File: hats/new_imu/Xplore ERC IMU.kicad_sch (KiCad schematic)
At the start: 42 parts, among them J1 5025850670, J2 5025850570, SW1 CAS-220TA, U1 LIS3MDL, U2 BMI088, U3 LT3960JMSE-PBF, U4 AMS1117-3.3, U5 D5V0H1B2LP-7B

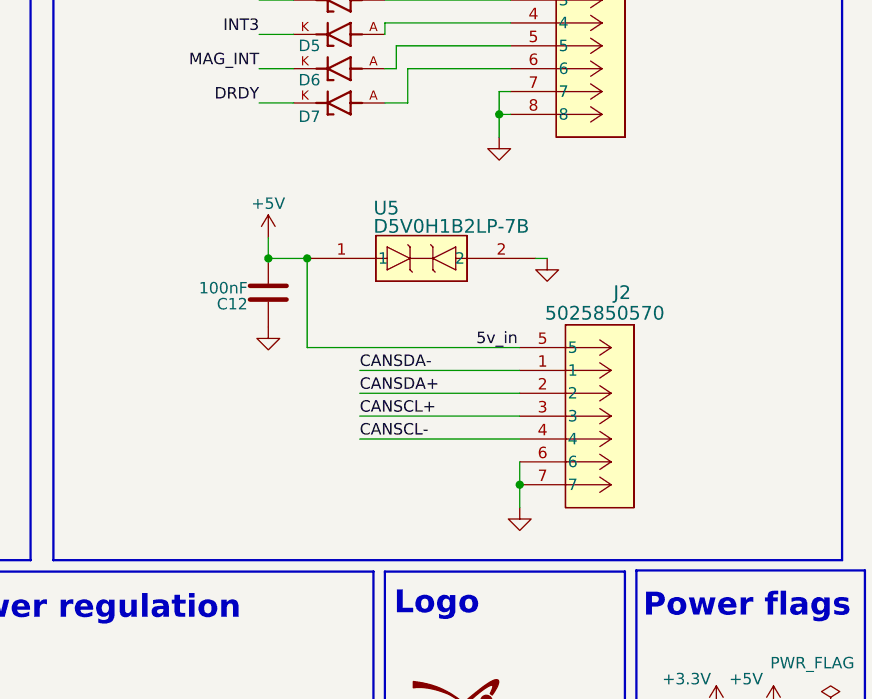
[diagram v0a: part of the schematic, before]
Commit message: IMU Layout and routing fixes
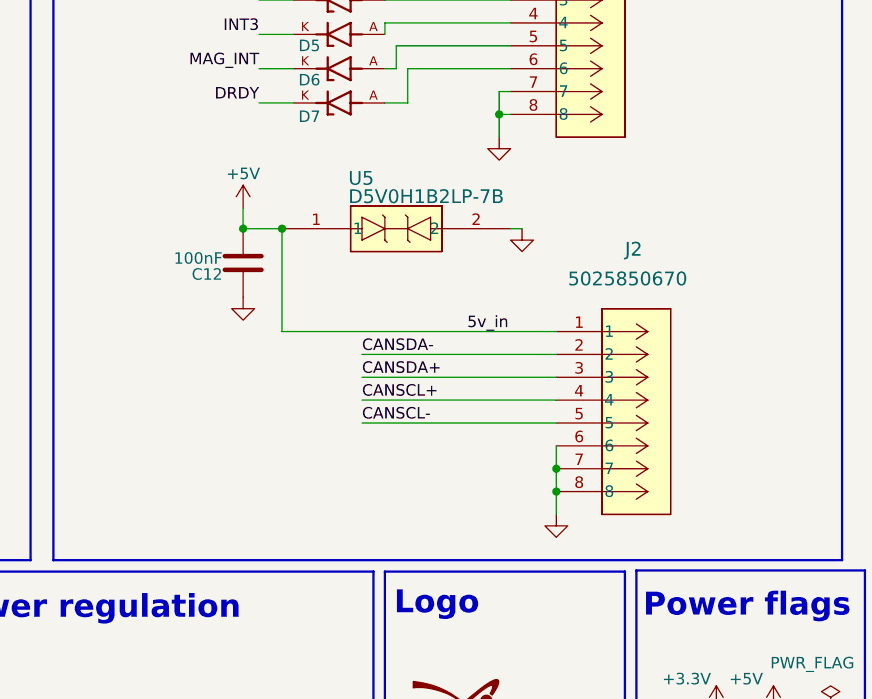
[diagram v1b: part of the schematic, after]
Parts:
- removed J2: 5025850570, footprints:CON_5025850570, symbol 5025850570:5025850570
- added J2: 5025850670, footprints:CON_5025850670, symbol 502585670:5025850670
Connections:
- net +5V: now also J2.1
- net CANSCL+: now also J2.4
- net CANSCL-: now also J2.5
- net CANSDA+: now also J2.3
- net CANSDA-: now also J2.2
- net GND: now also J2.6, J2.7, J2.8
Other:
- moved on the sheet: C12, U5

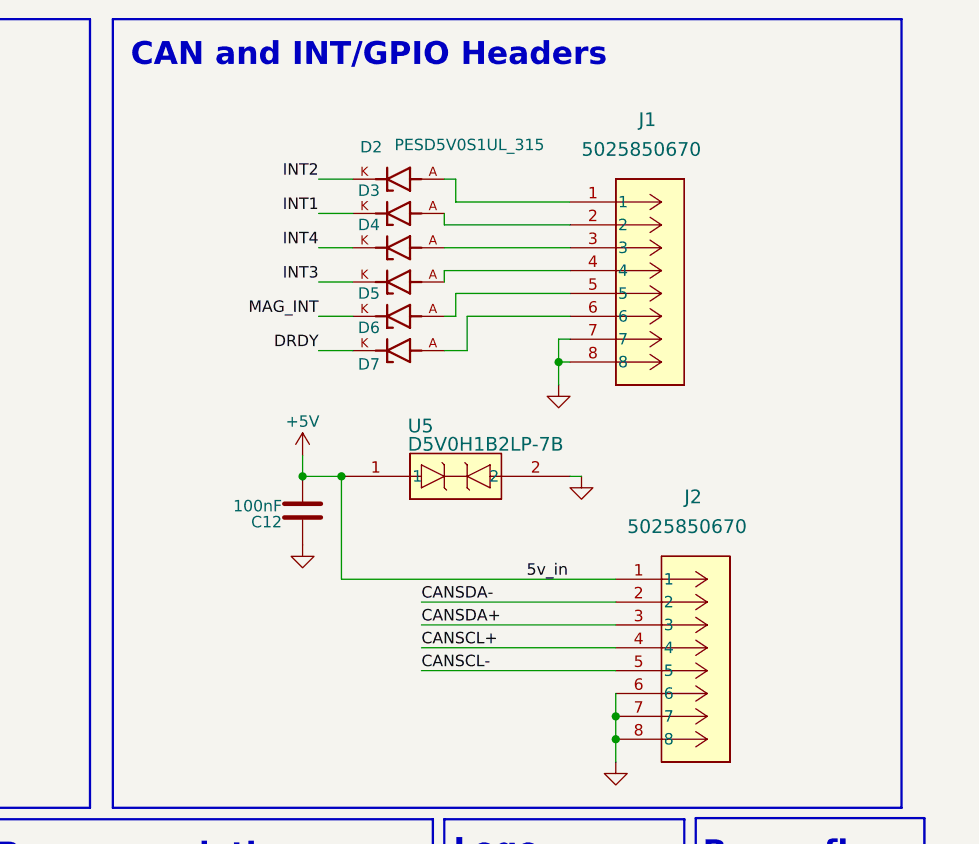
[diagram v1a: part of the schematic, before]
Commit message: IMU tweaks
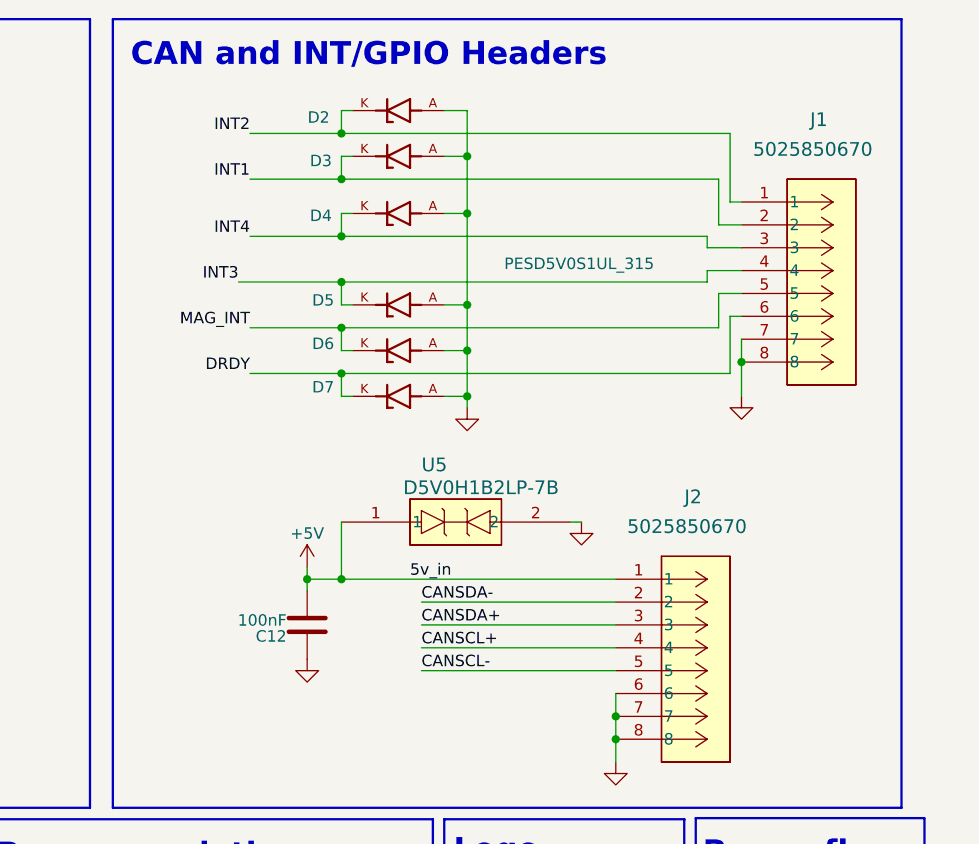
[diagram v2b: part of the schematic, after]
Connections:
- net DRDY: now also J1.6
- net GND: now also D2.A, D3.A, D4.A, D5.A, D6.A, D7.A
- net INT1: now also J1.2
- net INT2: now also J1.1
- net INT3: now also J1.4
- net INT4: now also J1.3
- net MAG_INT: now also J1.5
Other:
- moved on the sheet: C12, D3, D4, D5, D6, D7, J1, U5

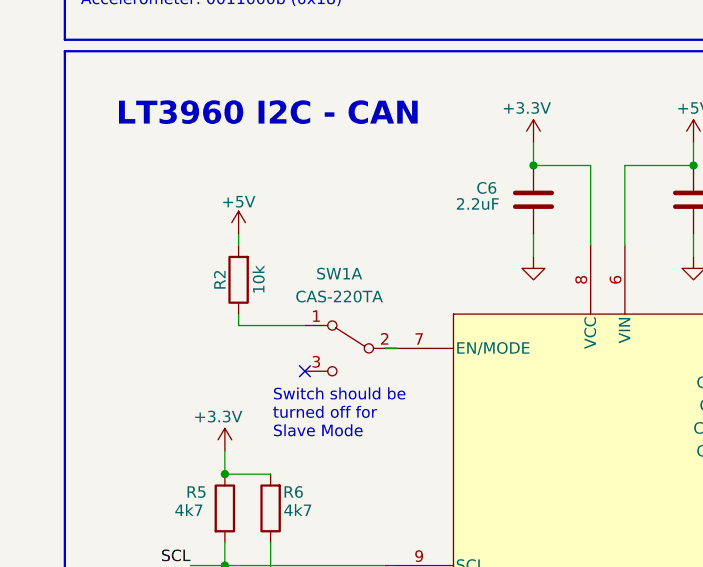
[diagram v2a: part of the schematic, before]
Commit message: IMU final touches
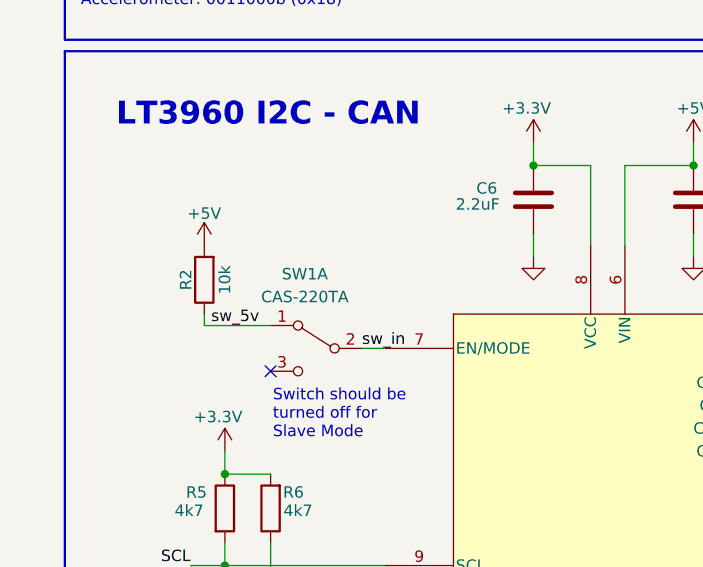
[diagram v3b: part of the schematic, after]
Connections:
- net sw_5v: now reaches R2.1, SW1.1 (A)
- net sw_in: now reaches SW1.2 (B), U3.7 (EN/MODE)
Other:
- moved on the sheet: R2, SW1A
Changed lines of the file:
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@@
 	)
 	(no_connect
-		(at 40.64 144.78)
+		(at 36.83 144.78)
 	)
 	(wire
@@
 	(wire
 		(pts
-			(xy 40.64 139.7) (xy 33.274 139.7)
+			(xy 36.83 139.7) (xy 29.464 139.7)
 		)
 		(stroke
@@
 	(wire
 		(pts
-			(xy 50.8 142.24) (xy 49.53 142.24)
-		)
-		(stroke
-			(width 0)
-			(type default)
-		)
-	)
-	(wire
-		(pts
 			(xy 100.33 148.59) (xy 104.14 148.59)
 		)
@@
 	(wire
 		(pts
-			(xy 33.274 139.7) (xy 33.274 138.43)
+			(xy 29.464 139.7) (xy 29.464 138.43)
 		)
 		(stroke
@@
 	(wire
 		(pts
+			(xy 46.99 142.24) (xy 49.53 142.24)
+		)
+		(stroke
+			(width 0)
+			(type default)
+		)
+	)
+	(wire
+		(pts
 			(xy 220.98 137.16) (xy 220.98 135.89)
 		)
@@
 	(wire
 		(pts
-			(xy 33.274 129.54) (xy 33.274 130.81)
-		)
-		(stroke
-			(width 0)
-			(type default)
-		)
-	)
-	(wire
-		(pts
 			(xy 262.89 33.02) (xy 262.89 40.64)
 		)
@@
 		)
 	)
+	(label "sw_in"
+		(at 46.99 142.24 0)
+		(fields_autoplaced yes)
+		(effects
+			(font
+				(size 1.27 1.27)
+			)
+			(justify left bottom)
+		)
+	)
+	(label "sw_5v"
+		(at 35.56 139.7 180)
+		(fields_autoplaced yes)
+		(effects
+			(font
+				(size 1.27 1.27)
+			)
+			(justify right bottom)
+		)
+	)
 	(label "MAG_INT"
 		(at 209.55 54.61 180)
@@
 	(symbol
 		(lib_id "power:+5V")
-		(at 33.274 129.54 0)
+		(at 29.464 130.81 0)
 		(unit 1)
 		(exclude_from_sim no)
@@
 		(dnp no)
 		(property "Reference" "#PWR019"
-			(at 33.274 133.35 0)
+			(at 29.464 134.62 0)
 			(effects
 				(font
@@
 		)
 		(property "Value" "+5V"
-			(at 33.274 125.984 0)
+			(at 29.464 127.254 0)
 			(effects
 				(font
@@
 		)
 		(property "Footprint" ""
-			(at 33.274 129.54 0)
+			(at 29.464 130.81 0)
 			(effects
 				(font
@@
 		)
 		(property "Datasheet" ""
-			(at 33.274 129.54 0)
+			(at 29.464 130.81 0)
 			(effects
 				(font
@@
 		)
 		(property "Description" "Power symbol creates a global label with name \"+5V\""
-			(at 33.274 129.54 0)
+			(at 29.464 130.81 0)
 			(effects
 				(font
@@
 	(symbol
 		(lib_id "Switch:SW_DPDT_x2")
-		(at 45.72 142.24 0)
+		(at 41.91 142.24 0)
 		(mirror y)
 		(unit 1)
@@
 		(dnp no)
 		(property "Reference" "SW1"
-			(at 44.45 133.985 0)
+			(at 40.64 133.985 0)
 			(effects
 				(font
@@
 		)
 		(property "Value" "CAS-220TA"
-			(at 44.45 136.525 0)
+			(at 40.64 136.525 0)
 			(effects
 				(font
@@
 		)
 		(property "Footprint" "0_switch_button:7M25000MAAJT"
-			(at 45.72 142.24 0)
+			(at 41.91 142.24 0)
 			(effects
 				(font
@@
 		)
 		(property "Datasheet" "https://www.nidec-copal-electronics.com/e/catalog/switch/cas.pdf"
-			(at 45.72 142.24 0)
+			(at 41.91 142.24 0)
 			(effects
 				(font
@@
 		)
 		(property "Description" "SWITCH SLIDE DPDT 100MA 6V"
-			(at 45.72 142.24 0)
+			(at 41.91 142.24 0)
 			(effects
 				(font
@@
 		)
 		(property "Manufacturer Part Number" "CAS-220TA"
-			(at 45.72 142.24 0)
+			(at 41.91 142.24 0)
 			(effects
 				(font
@@
 		)
 		(property "Supplier 1" "Digikey"
-			(at 45.72 142.24 0)
+			(at 41.91 142.24 0)
 			(effects
 				(font
@@
 		)
 		(property "Supplier Part Number 1" "CAS220JCT-ND"
-			(at 45.72 142.24 0)
+			(at 41.91 142.24 0)
 			(effects
 				(font
@@
 		)
 		(property "Manufacturer" "Nidec Components Corporation"
-			(at 45.72 142.24 0)
+			(at 41.91 142.24 0)
 			(effects
 				(font
@@
 	(symbol
 		(lib_id "Device:R")
-		(at 33.274 134.62 180)
+		(at 29.464 134.62 180)
 		(unit 1)
 		(exclude_from_sim no)
@@
 		(dnp no)
 		(property "Reference" "R2"
-			(at 31.242 134.62 90)
+			(at 27.432 134.62 90)
 			(effects
 				(font
@@
 		)
 		(property "Value" "10k"
-			(at 35.56 134.62 90)
+			(at 31.75 134.62 90)
 			(effects
 				(font
@@
 		)
 		(property "Footprint" "Resistor_SMD:R_0402_1005Metric"
-			(at 35.052 134.62 90)
+			(at 31.242 134.62 90)
 			(effects
 				(font
@@
 		)
 		(property "Datasheet" "~"
-			(at 33.274 134.62 0)
+			(at 29.464 134.62 0)
 			(effects
 				(font
@@
 		)
 		(property "Description" "Resistor"
-			(at 33.274 134.62 0)
+			(at 29.464 134.62 0)
 			(effects
 				(font

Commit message: IMU final touches
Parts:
- SW1: footprint 0_switch_button:7M25000MAAJT -> 0_switch_button:CAS-220A_NDC
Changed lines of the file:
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@@
 			)
 		)
-		(property "Footprint" "0_switch_button:7M25000MAAJT"
+		(property "Footprint" "0_switch_button:CAS-220A_NDC"
 			(at 41.91 142.24 0)
 			(effects

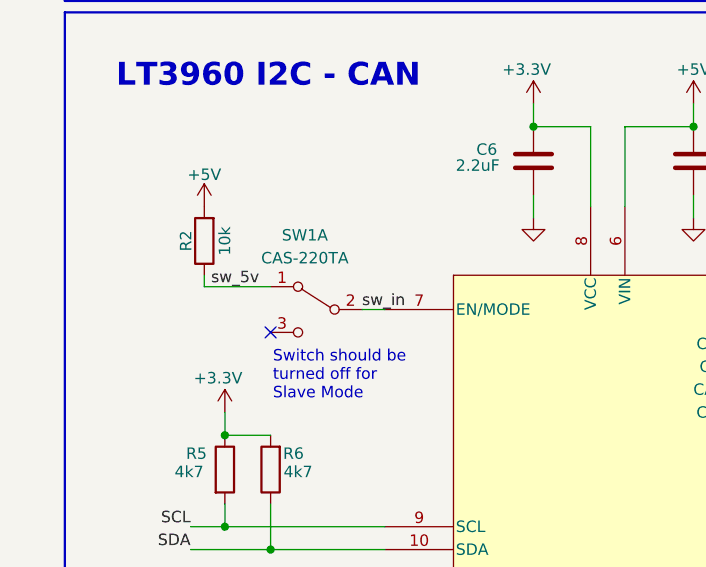
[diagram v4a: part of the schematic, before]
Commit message: Corrected some things, still need top check impedance control
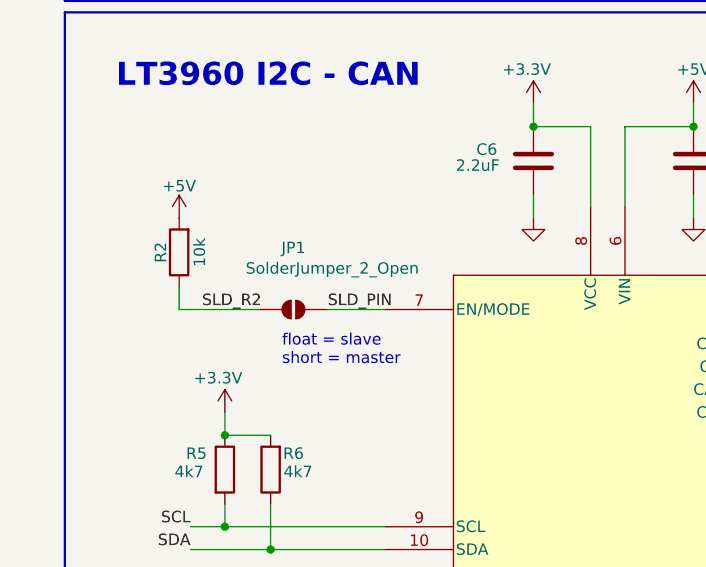
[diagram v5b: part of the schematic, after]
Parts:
- removed SW1: CAS-220TA, 0_switch_button:CAS-220A_NDC, symbol Switch:SW_DPDT_x2
- added JP1: SolderJumper_2_Open, Jumper:SolderJumper-2_P1.3mm_Open_RoundedPad1.0x1.5mm, symbol Jumper:SolderJumper_2_Open
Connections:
- net sw_5v renamed SLD_R2
- net SLD_R2: now also JP1.1 (A)
- net sw_in renamed SLD_PIN
- net SLD_PIN: now also JP1.2 (B)
- no-connect marks 2 -> 1
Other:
- note added: "float = slave short = master"
- note removed: "Switch should be turned off for Slave Mode"
- moved on the sheet: R2
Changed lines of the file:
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@@
 		(at 38.1 67.31)
 	)
-	(no_connect
-		(at 36.83 144.78)
-	)
 	(wire
 		(pts
@@
 	(wire
 		(pts
-			(xy 36.83 139.7) (xy 29.464 139.7)
-		)
-		(stroke
-			(width 0)
-			(type default)
-		)
-	)
-	(wire
-		(pts
 			(xy 231.14 35.56) (xy 233.68 35.56)
 		)
@@
 	(wire
 		(pts
-			(xy 29.464 139.7) (xy 29.464 138.43)
-		)
-		(stroke
-			(width 0)
-			(type default)
-		)
-	)
-	(wire
-		(pts
 			(xy 219.71 35.56) (xy 220.98 35.56)
 		)
@@
 	(wire
 		(pts
-			(xy 46.99 142.24) (xy 49.53 142.24)
+			(xy 43.18 142.24) (xy 49.53 142.24)
 		)
 		(stroke
@@
 	(wire
 		(pts
+			(xy 26.67 142.24) (xy 26.67 139.7)
+		)
+		(stroke
+			(width 0)
+			(type default)
+		)
+	)
+	(wire
+		(pts
 			(xy 220.98 149.86) (xy 220.98 151.13)
 		)
@@
 	(wire
 		(pts
+			(xy 26.67 142.24) (xy 35.56 142.24)
+		)
+		(stroke
+			(width 0)
+			(type default)
+		)
+	)
+	(wire
+		(pts
 			(xy 228.6 90.17) (xy 250.19 90.17)
 		)
@@
 		)
 	)
-	(text "Switch should be \nturned off for \nSlave Mode\n"
+	(text "float = slave\nshort = master\n"
 		(exclude_from_sim no)
-		(at 37.084 149.606 0)
+		(at 38.1 146.812 0)
 		(effects
 			(font
@@
 		)
 	)
+	(label "SLD_PIN"
+		(at 43.18 142.24 0)
+		(fields_autoplaced yes)
+		(effects
+			(font
+				(size 1.27 1.27)
+			)
+			(justify left bottom)
+		)
+	)
 	(label "MAG_INT"
 		(at 154.94 66.04 0)
@@
 		)
 	)
-	(label "SDA"
-		(at 124.46 72.39 0)
-		(fields_autoplaced yes)
-		(effects
-			(font
-				(size 1.27 1.27)
-			)
-			(justify left bottom)
-		)
-	)
-	(label "INT4"
-		(at 73.66 77.47 0)
+	(label "SLD_R2"
+		(at 29.21 142.24 0)
 		(fields_autoplaced yes)
 		(effects
@@
 	)
 	(label "SDA"
-		(at 27.94 168.91 180)
+		(at 124.46 72.39 0)
 		(fields_autoplaced yes)
 		(effects
@@
 				(size 1.27 1.27)
 			)
-			(justify right bottom)
+			(justify left bottom)
 		)
 	)
-	(label "sw_in"
-		(at 46.99 142.24 0)
+	(label "INT4"
+		(at 73.66 77.47 0)
 		(fields_autoplaced yes)
 		(effects
@@
 		)
 	)
-	(label "sw_5v"
-		(at 35.56 139.7 180)
+	(label "SDA"
+		(at 27.94 168.91 180)
 		(fields_autoplaced yes)
 		(effects
@@
 	(symbol
 		(lib_id "power:+5V")
-		(at 29.464 130.81 0)
+		(at 26.67 132.08 0)
 		(unit 1)
 		(exclude_from_sim no)
@@
 		(dnp no)
 		(property "Reference" "#PWR019"
-			(at 29.464 134.62 0)
+			(at 26.67 135.89 0)
 			(effects
 				(font
@@
 		)
 		(property "Value" "+5V"
-			(at 29.464 127.254 0)
+			(at 26.67 128.524 0)
 			(effects
 				(font
@@
 		)
 		(property "Footprint" ""
-			(at 29.464 130.81 0)
+			(at 26.67 132.08 0)
 			(effects
 				(font
@@
 		)
 		(property "Datasheet" ""
-			(at 29.464 130.81 0)
+			(at 26.67 132.08 0)
 			(effects
 				(font
@@
 		)
 		(property "Description" "Power symbol creates a global label with name \"+5V\""
-			(at 29.464 130.81 0)
+			(at 26.67 132.08 0)
 			(effects
 				(font
@@
 	)
 	(symbol
-		(lib_id "Switch:SW_DPDT_x2")
-		(at 41.91 142.24 0)
-		(mirror y)
-		(unit 1)
-		(exclude_from_sim no)
-		(in_bom yes)
-		(on_board yes)
-		(dnp no)
-		(property "Reference" "SW1"
-			(at 40.64 133.985 0)
-			(effects
-				(font
-					(size 1.27 1.27)
-				)
-			)
-		)
-		(property "Value" "CAS-220TA"
-			(at 40.64 136.525 0)
-			(effects
-				(font
-					(size 1.27 1.27)
-				)
-			)
-		)
-		(property "Footprint" "0_switch_button:CAS-220A_NDC"
-			(at 41.91 142.24 0)
-			(effects
-				(font
-					(size 1.27 1.27)
-				)
-				(hide yes)
-			)
-		)
-		(property "Datasheet" "https://www.nidec-copal-electronics.com/e/catalog/switch/cas.pdf"
-			(at 41.91 142.24 0)
-			(effects
-				(font
-					(size 1.27 1.27)
-				)
-				(hide yes)
-			)
-		)
-		(property "Description" "SWITCH SLIDE DPDT 100MA 6V"
-			(at 41.91 142.24 0)
-			(effects
-				(font
-					(size 1.27 1.27)
-				)
-				(hide yes)
-			)
-		)
-		(property "Manufacturer Part Number" "CAS-220TA"
-			(at 41.91 142.24 0)
-			(effects
-				(font
-					(size 1.27 1.27)
-				)
-				(hide yes)
-			)
-		)
-		(property "Supplier 1" "Digikey"
-			(at 41.91 142.24 0)
-			(effects
-				(font
-					(size 1.27 1.27)
-				)
-				(hide yes)
-			)
-		)
-		(property "Supplier Part Number 1" "CAS220JCT-ND"
-			(at 41.91 142.24 0)
-			(effects
-				(font
-					(size 1.27 1.27)
-				)
-				(hide yes)
-			)
-		)
-		(property "Manufacturer" "Nidec Components Corporation"
-			(at 41.91 142.24 0)
-			(effects
-				(font
-					(size 1.27 1.27)
-				)
-				(hide yes)
-			)
-		)
-		(pin "1"
-		)
-		(pin "2"
-		)
-		(pin "3"
-		)
-		(pin "4"
-		)
-		(pin "5"
-		)
-		(pin "6"
-		)
-		(instances
-			(project "Xplore ERC IMU"
-				(path "/52d76c23-ecf1-4115-8362-f772e097cafa"
-					(reference "SW1")
-					(unit 1)
-				)
-			)
-		)
-	)
-	(symbol
 		(lib_id "Device:R_Small")
 		(at 220.98 139.7 180)
@@
 	(symbol
 		(lib_id "Device:R")
-		(at 29.464 134.62 180)
+		(at 26.67 135.89 180)
 		(unit 1)
 		(exclude_from_sim no)
@@
 		(dnp no)
 		(property "Reference" "R2"
-			(at 27.432 134.62 90)
+			(at 24.638 135.89 90)
 			(effects
 				(font
@@
 		)
 		(property "Value" "10k"
-			(at 31.75 134.62 90)
+			(at 28.956 135.89 90)
 			(effects
 				(font
@@
 		)
 		(property "Footprint" "Resistor_SMD:R_0402_1005Metric"
-			(at 31.242 134.62 90)
+			(at 28.448 135.89 90)
 			(effects
 				(font
@@
 		)
 		(property "Datasheet" "~"
-			(at 29.464 134.62 0)
+			(at 26.67 135.89 0)
 			(effects
 				(font
@@
 		)
 		(property "Description" "Resistor"
-			(at 29.464 134.62 0)
+			(at 26.67 135.89 0)
 			(effects
 				(font
@@
 					(unit 1)
 				)
+			)
+		)
+	)
+	(symbol
+		(lib_id "Jumper:SolderJumper_2_Open")
+		(at 39.37 142.24 0)
+		(unit 1)
+		(exclude_from_sim yes)
+		(in_bom no)
+		(on_board yes)
+		(dnp no)
+		(property "Reference" "JP1"
+			(at 39.37 135.382 0)
+			(effects
+				(font
+					(size 1.27 1.27)
+				)
+			)
+		)
+		(property "Value" "SolderJumper_2_Open"
+			(at 43.688 137.668 0)
+			(effects
+				(font
+					(size 1.27 1.27)
+				)
+			)
+		)
+		(property "Footprint" "Jumper:SolderJumper-2_P1.3mm_Open_RoundedPad1.0x1.5mm"
+			(at 39.37 142.24 0)
+			(effects
+				(font
+					(size 1.27 1.27)
+				)
+				(hide yes)
+			)
+		)
+		(property "Datasheet" "~"
+			(at 39.37 142.24 0)
+			(effects
+				(font
+					(size 1.27 1.27)
+				)
+				(hide yes)
+			)
+		)
+		(property "Description" "Solder Jumper, 2-pole, open"
+			(at 39.37 142.24 0)
+			(effects
+				(font
+					(size 1.27 1.27)
+				)
+				(hide yes)
+			)
+		)
+		(pin "1"
+		)
+		(pin "2"
+		)
+		(instances
+			(project ""
+				(path "/52d76c23-ecf1-4115-8362-f772e097cafa"
+					(reference "JP1")
+					(unit 1)
+				)

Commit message: changed the capas to bigger ones as Ismail did before
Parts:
- C10, C11: footprint Capacitor_SMD:C_0402_1005Metric -> Capacitor_SMD:C_0805_2012Metric
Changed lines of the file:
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@@
 			)
 		)
-		(property "Footprint" "Capacitor_SMD:C_0402_1005Metric"
+		(property "Footprint" "Capacitor_SMD:C_0805_2012Metric"
 			(at 210.5152 147.32 0)
 			(effects
@@
 			)
 		)
-		(property "Footprint" "Capacitor_SMD:C_0402_1005Metric"
+		(property "Footprint" "Capacitor_SMD:C_0805_2012Metric"
 			(at 183.8452 147.32 0)
 			(effects
